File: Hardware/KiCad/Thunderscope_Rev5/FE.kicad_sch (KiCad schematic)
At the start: 23 parts, among them Q1 DMN62D0UW, Q2 DMN62D0UW, U2 MCP4452-104E, U3 MCP4728, U4 REF2025, U5 OPA140AIDR

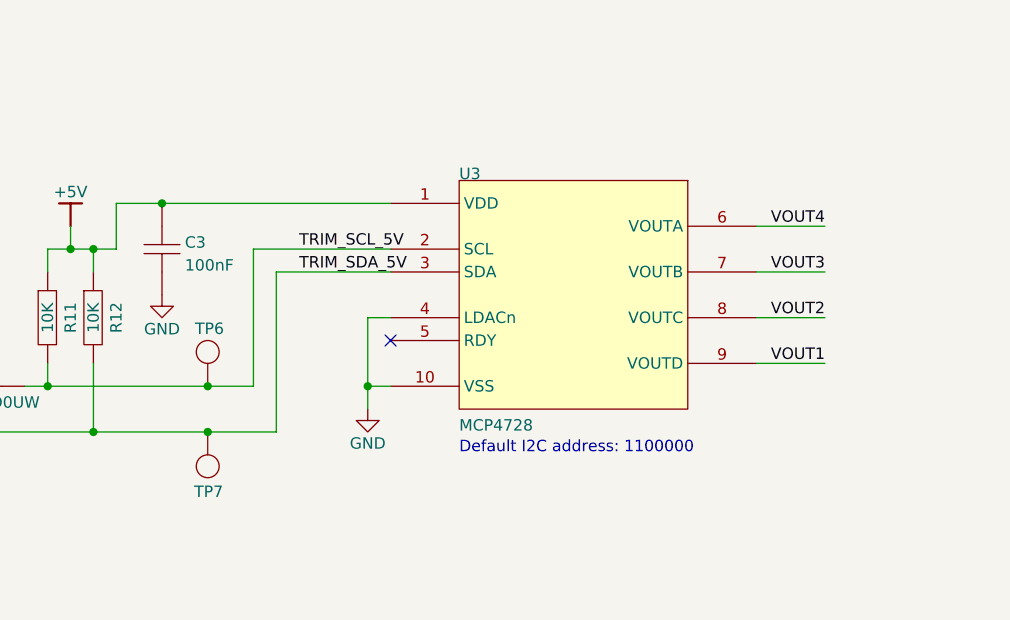
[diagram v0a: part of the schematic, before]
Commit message: Refactored Schematic
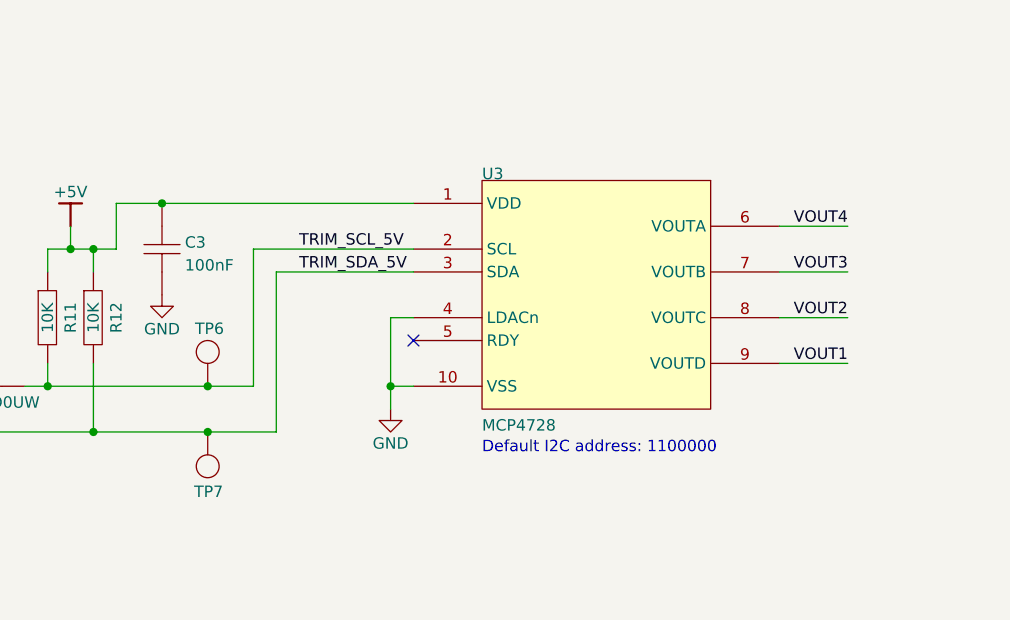
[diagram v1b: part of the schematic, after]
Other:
- moved on the sheet: U3
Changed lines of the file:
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@@
 	(text "Default I2C address: 1100000"
 		(exclude_from_sim no)
-		(at 121.92 71.12 0)
+		(at 124.46 71.12 0)
 		(effects
 			(font
@@
 	)
 	(junction
-		(at 111.76 63.5)
+		(at 114.3 63.5)
 		(diameter 0)
 		(color 0 0 0 0)
@@
 	)
 	(no_connect
-		(at 114.3 58.42)
+		(at 116.84 58.42)
 	)
 	(no_connect
@@
 	(wire
 		(pts
-			(xy 114.3 63.5) (xy 111.76 63.5)
+			(xy 116.84 63.5) (xy 114.3 63.5)
 		)
 		(stroke
@@
 	(wire
 		(pts
-			(xy 88.9 43.18) (xy 114.3 43.18)
+			(xy 88.9 43.18) (xy 116.84 43.18)
 		)
 		(stroke
@@
 	(wire
 		(pts
-			(xy 154.94 55.88) (xy 162.56 55.88)
+			(xy 157.48 55.88) (xy 165.1 55.88)
 		)
 		(stroke
@@
 	(wire
 		(pts
-			(xy 114.3 55.88) (xy 111.76 55.88)
+			(xy 116.84 55.88) (xy 114.3 55.88)
 		)
 		(stroke
@@
 	(wire
 		(pts
-			(xy 99.06 48.26) (xy 114.3 48.26)
+			(xy 99.06 48.26) (xy 116.84 48.26)
 		)
 		(stroke
@@
 	(wire
 		(pts
-			(xy 154.94 50.8) (xy 162.56 50.8)
+			(xy 157.48 50.8) (xy 165.1 50.8)
 		)
 		(stroke
@@
 	(wire
 		(pts
-			(xy 154.94 60.96) (xy 162.56 60.96)
+			(xy 157.48 60.96) (xy 165.1 60.96)
 		)
 		(stroke
@@
 	(wire
 		(pts
-			(xy 111.76 63.5) (xy 111.76 66.04)
+			(xy 114.3 63.5) (xy 114.3 66.04)
 		)
 		(stroke
@@
 	(wire
 		(pts
-			(xy 101.6 50.8) (xy 114.3 50.8)
+			(xy 101.6 50.8) (xy 116.84 50.8)
 		)
 		(stroke
@@
 	(wire
 		(pts
-			(xy 111.76 55.88) (xy 111.76 63.5)
+			(xy 114.3 55.88) (xy 114.3 63.5)
 		)
 		(stroke
@@
 	(wire
 		(pts
-			(xy 154.94 45.72) (xy 162.56 45.72)
+			(xy 157.48 45.72) (xy 165.1 45.72)
 		)
 		(stroke
@@
 	)
 	(label "VOUT3"
-		(at 162.56 50.8 180)
+		(at 165.1 50.8 180)
 		(effects
 			(font
@@
 	)
 	(label "VOUT4"
-		(at 162.56 45.72 180)
+		(at 165.1 45.72 180)
 		(effects
 			(font
@@
 	)
 	(label "VOUT2"
-		(at 162.56 55.88 180)
+		(at 165.1 55.88 180)
 		(effects
 			(font
@@
 	)
 	(label "VOUT1"
-		(at 162.56 60.96 180)
+		(at 165.1 60.96 180)
 		(effects
 			(font
@@
 	(symbol
 		(lib_id "Thunderscope_Rev5:IC DAC QUAD MCP4728")
-		(at 134.62 53.34 0)
+		(at 137.16 53.34 0)
 		(unit 1)
 		(exclude_from_sim no)
@@
 		(dnp no)
 		(property "Reference" "U3"
-			(at 121.92 40.64 0)
+			(at 124.46 40.64 0)
 			(effects
 				(font
@@
 		)
 		(property "Value" "MCP4728"
-			(at 121.92 68.58 0)
+			(at 124.46 68.58 0)
 			(effects
 				(font
@@
 		)
 		(property "Footprint" "Thunderscope_Rev5:MC_MSOP10_UN"
-			(at 134.62 53.34 0)
+			(at 137.16 53.34 0)
 			(effects
 				(font
@@
 		)
 		(property "Datasheet" ""
-			(at 134.62 53.34 0)
+			(at 137.16 53.34 0)
 			(effects
 				(font
@@
 		)
 		(property "Description" ""
-			(at 134.62 53.34 0)
+			(at 137.16 53.34 0)
 			(effects
 				(font
@@
 		)
 		(property "SUPPLIER 1" "Mouser"
-			(at 133.35 52.07 0)
+			(at 135.89 52.07 0)
 			(effects
 				(font
@@
 		)
 		(property "SUPPLIER PART NUMBER 1" "579-MCP4728A1T-E/UN"
-			(at 133.35 52.07 0)
+			(at 135.89 52.07 0)
 			(effects
 				(font
@@
 		)
 		(property "HOUSE PART NUMBER" ""
-			(at 113.792 38.1 0)
+			(at 116.332 38.1 0)
 			(effects
 				(font
@@
 		)
 		(property "MANUFACTURER" "Microchip"
-			(at 113.792 38.1 0)
+			(at 116.332 38.1 0)
 			(effects
 				(font
@@
 		)
 		(property "MANUFACTURER PART NUMBER" "MCP4728"
-			(at 113.792 38.1 0)
+			(at 116.332 38.1 0)
 			(effects
 				(font
@@
 		)
 		(property "ALTIUM_VALUE" ""
-			(at 134.62 53.34 0)
+			(at 137.16 53.34 0)
 			(effects
 				(font
@@
 	(symbol
 		(lib_id "Thunderscope_Rev5:GND")
-		(at 111.76 66.04 0)
+		(at 114.3 66.04 0)
 		(unit 1)
 		(exclude_from_sim no)
@@
 		(dnp no)
 		(property "Reference" "#PWR0181"
-			(at 111.76 72.39 0)
+			(at 114.3 72.39 0)
 			(effects
 				(font
@@
 		)
 		(property "Value" "GND"
-			(at 111.76 69.85 0)
+			(at 114.3 69.85 0)
 			(effects
 				(font
@@
 		)
 		(property "Footprint" ""
-			(at 111.76 66.04 0)
+			(at 114.3 66.04 0)
 			(effects
 				(font
@@
 		)
 		(property "Datasheet" ""
-			(at 111.76 66.04 0)
+			(at 114.3 66.04 0)
 			(effects
 				(font
@@
 		)
 		(property "Description" "Power symbol creates a global label with name \"GND\" , ground"
-			(at 111.76 66.04 0)
+			(at 114.3 66.04 0)
 			(effects
 				(font
